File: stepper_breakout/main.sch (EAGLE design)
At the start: 36 parts, among them J1 XH_4POS_DEV, J10 3_PIN_SCREW_3.5MM_DEV, J11 3_PIN_SCREW_3.5MM_DEV, J12 2_PIN_SCREW_3.5MM_DEV, J13 4_PIN_2.54MM_PKG, J2 XH_4POS_DEV, J3 XH_4POS_DEV, J4 XH_4POS_DEV, J5 XH_4POS_DEV, J6 XH_3POS_DEV, J7 XH_3POS_DEV, J8 XH_3POS_DEV, J9 3_PIN_SCREW_3.5MM_DEV, U1 ESP32_WROOM_BREAKOUT_DEV, U2 8_CHANNEL_LEVEL_SHIFTER, U3 5V_SWITCHING_POWER_DEV, U4 MAX_485_DEV

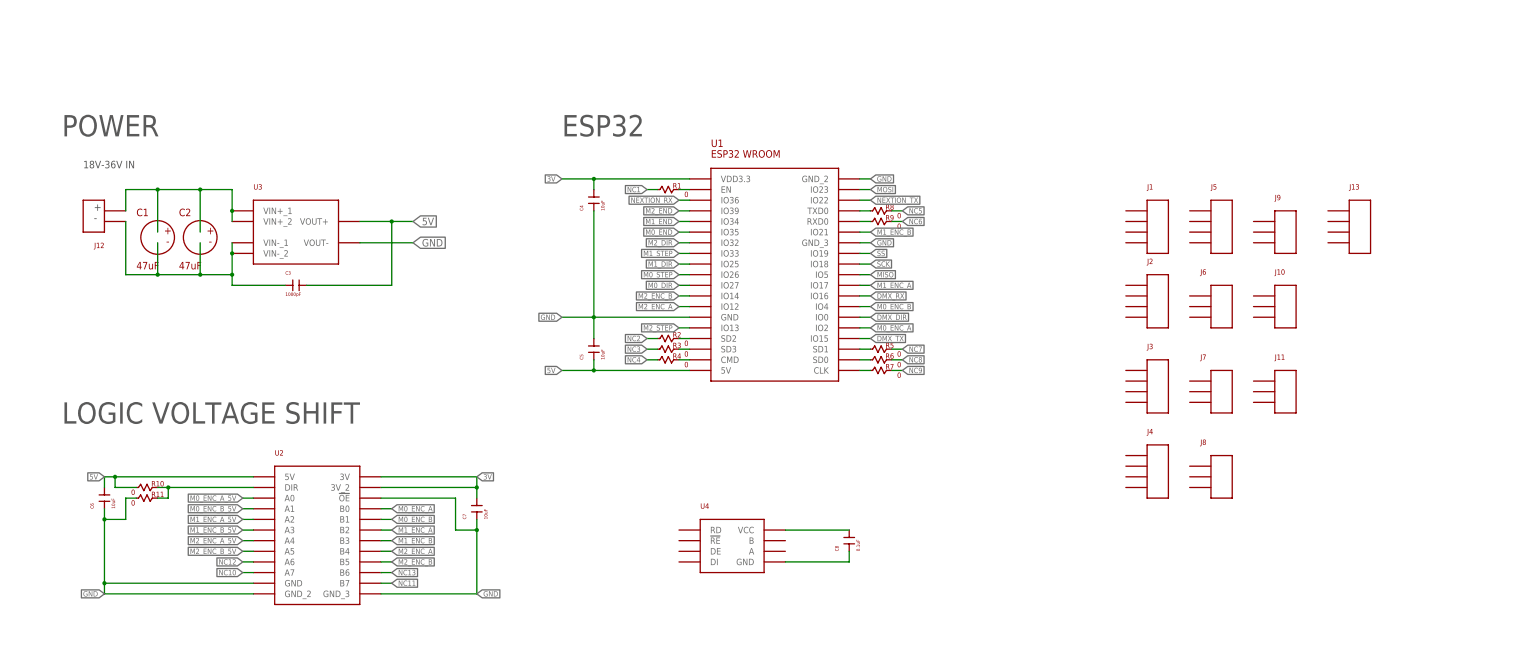
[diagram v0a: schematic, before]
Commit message: rev1 done
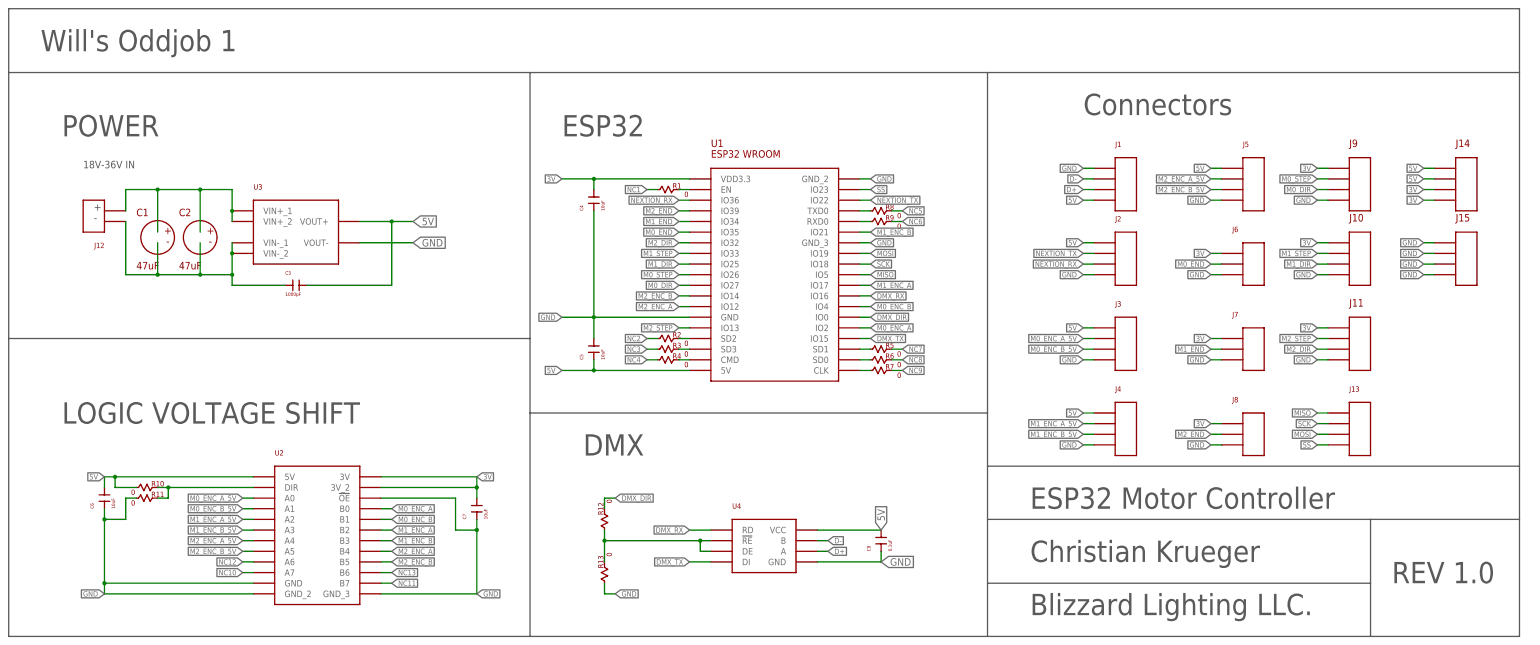
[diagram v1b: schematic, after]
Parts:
- added J14, J15: 4_PIN_SCREW_3.5MM_DEV, blizzard_common_0:4_PIN_SCREW_3.5MM_DEV
- added R12, R13: 0, blizzard_common_1:0805_RES_DEV
- J10, J11, J9: value 3_PIN_SCREW_3.5MM_DEV -> 4_PIN_SCREW_3.5MM_DEV; device blizzard_common_0:3_PIN_SCREW_3.5MM_DEV -> blizzard_common_0:4_PIN_SCREW_3.5MM_DEV
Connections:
- removed net N$8: C8.P$1, U4.GND
- new net D+: J1.P$3, U4.A
- new net D-: J1.P$2, U4.B
- net 3V: now also J10.P$1, J11.P$1, J14.P$3, J14.P$4, J6.1, J7.1, J8.1, J9.P$1
- net 5V: now also C8.P$2, J1.P$4, J14.P$1, J14.P$2, J2.P$1, J3.P$1, J4.P$1, J5.P$1, U4.VCC
- net DMX_DIR: now also R12.P$2
- net DMX_RX: now also U4.RD
- net DMX_TX: now also U4.DI
- net GND: now also C8.P$1, J1.P$1, J10.P$4, J11.P$4, J15.P$1, J15.P$2, J15.P$3, J15.P$4, J2.P$4, J3.P$4, J4.P$4, J5.P$4, J6.3, J7.3, J8.3, J9.P$4, R13.P$1, U4.GND
- net M0_DIR: now also J9.P$3
- net M0_ENC_A_5V: now also J3.P$2
- net M0_ENC_B_5V: now also J3.P$3
- net M0_END: now also J6.2
- net M0_STEP: now also J9.P$2
- net M1_DIR: now also J10.P$3
- net M1_ENC_A_5V: now also J4.P$2
- net M1_ENC_B_5V: now also J4.P$3
- net M1_END: now also J7.2
- net M1_STEP: now also J10.P$2
- net M2_DIR: now also J11.P$3
- net M2_ENC_A_5V: now also J5.P$2
- net M2_ENC_B_5V: now also J5.P$3
- net M2_END: now also J8.2
- net M2_STEP: now also J11.P$2
- net MISO: now also J13.1
- net MOSI: now also J13.3, U1.IO19; no longer U1.IO23
- net N$4: now also R12.P$1, R13.P$2, U4.!RE, U4.DE; no longer C8.P$2, U4.VCC
- net NEXTION_RX: now also J2.P$3
- net NEXTION_TX: now also J2.P$2
- net SCK: now also J13.2
- net SS: now also J13.4, U1.IO23; no longer U1.IO19
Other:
- note added: "Blizzard Lighting LLC."
- note added: "Christian Krueger"
- note added: "Connectors"
- note added: "DMX"
- note added: "ESP32 Motor Controller"
- note added: "REV 1.0"
- note added: "Will's Oddjob 1"
- moved on the sheet: C8, J1, J13, J2, J3, J4, J5, J6, J7, J8, U4
